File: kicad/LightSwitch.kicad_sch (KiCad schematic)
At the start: 33 parts, among them J1 Screw_Terminal_01x02, J2 Conn_01x06_Female, J3 Conn_ARM_JTAG_SWD_10, J4 Conn_ARM_JTAG_SWD_10, Q1 MMBT2222A, Q2 MMBT2222A, SW1 SW_Push_LED, SW2 SW_Push_LED, SW3 SW_Push_LED, SW4 SW_Push_LED, SW5 SW_Push_LED, U1 LM2936-3.0, U2 SHT35-DIS, U3 E73-2G4M08S1C, U4 MX25R3235FM2xx0, Y1 32.768kHz

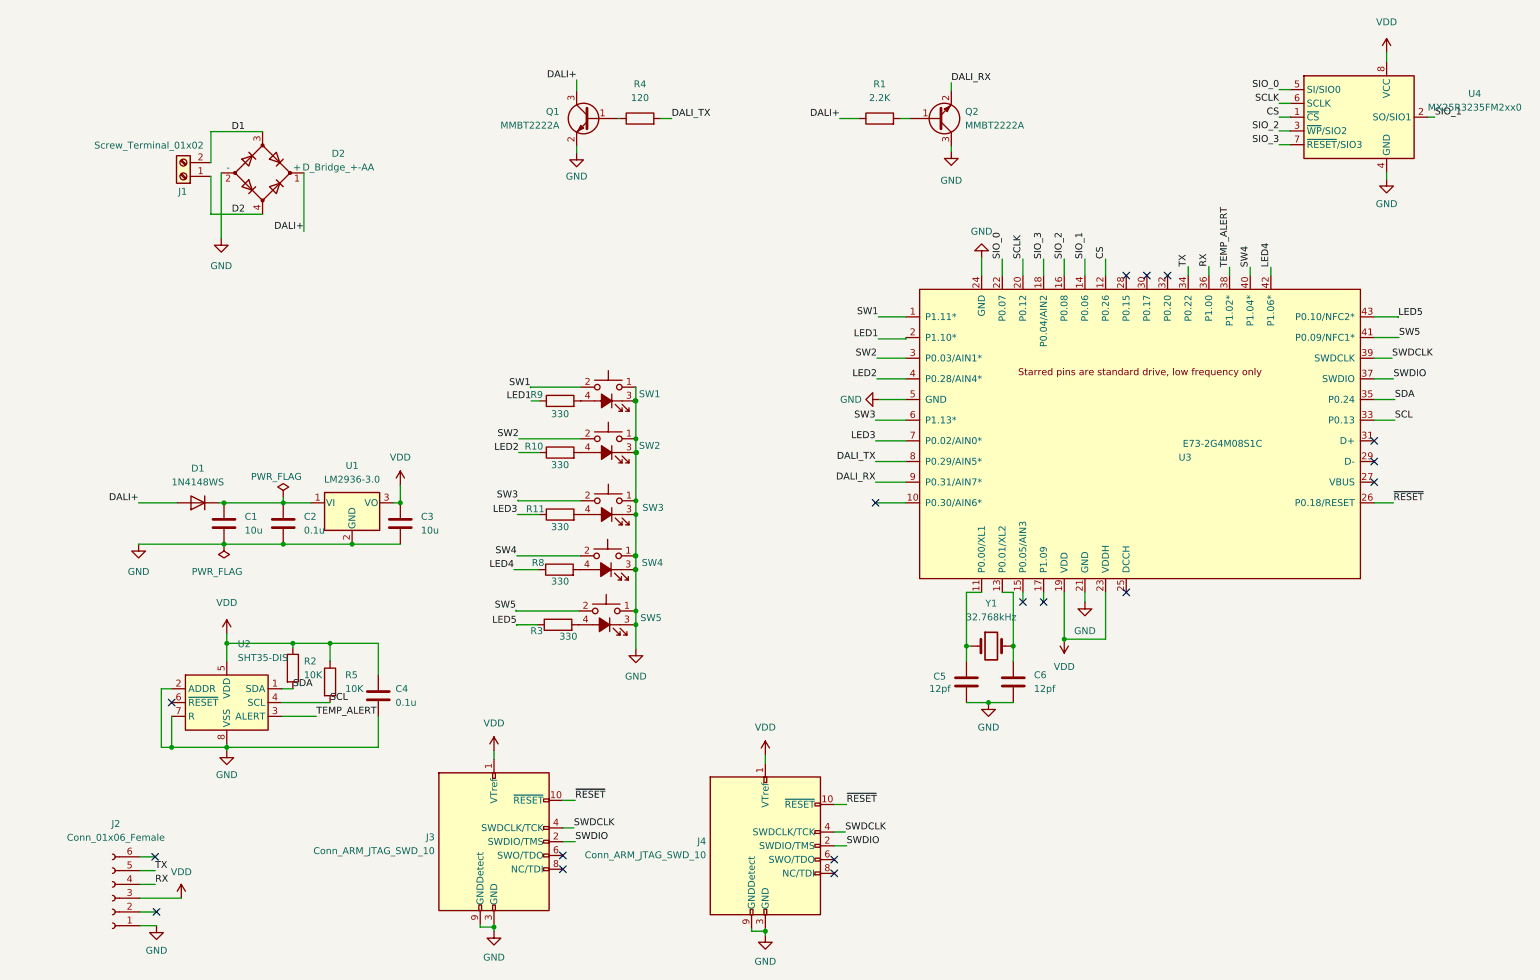
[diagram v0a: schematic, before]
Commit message: latect schematic
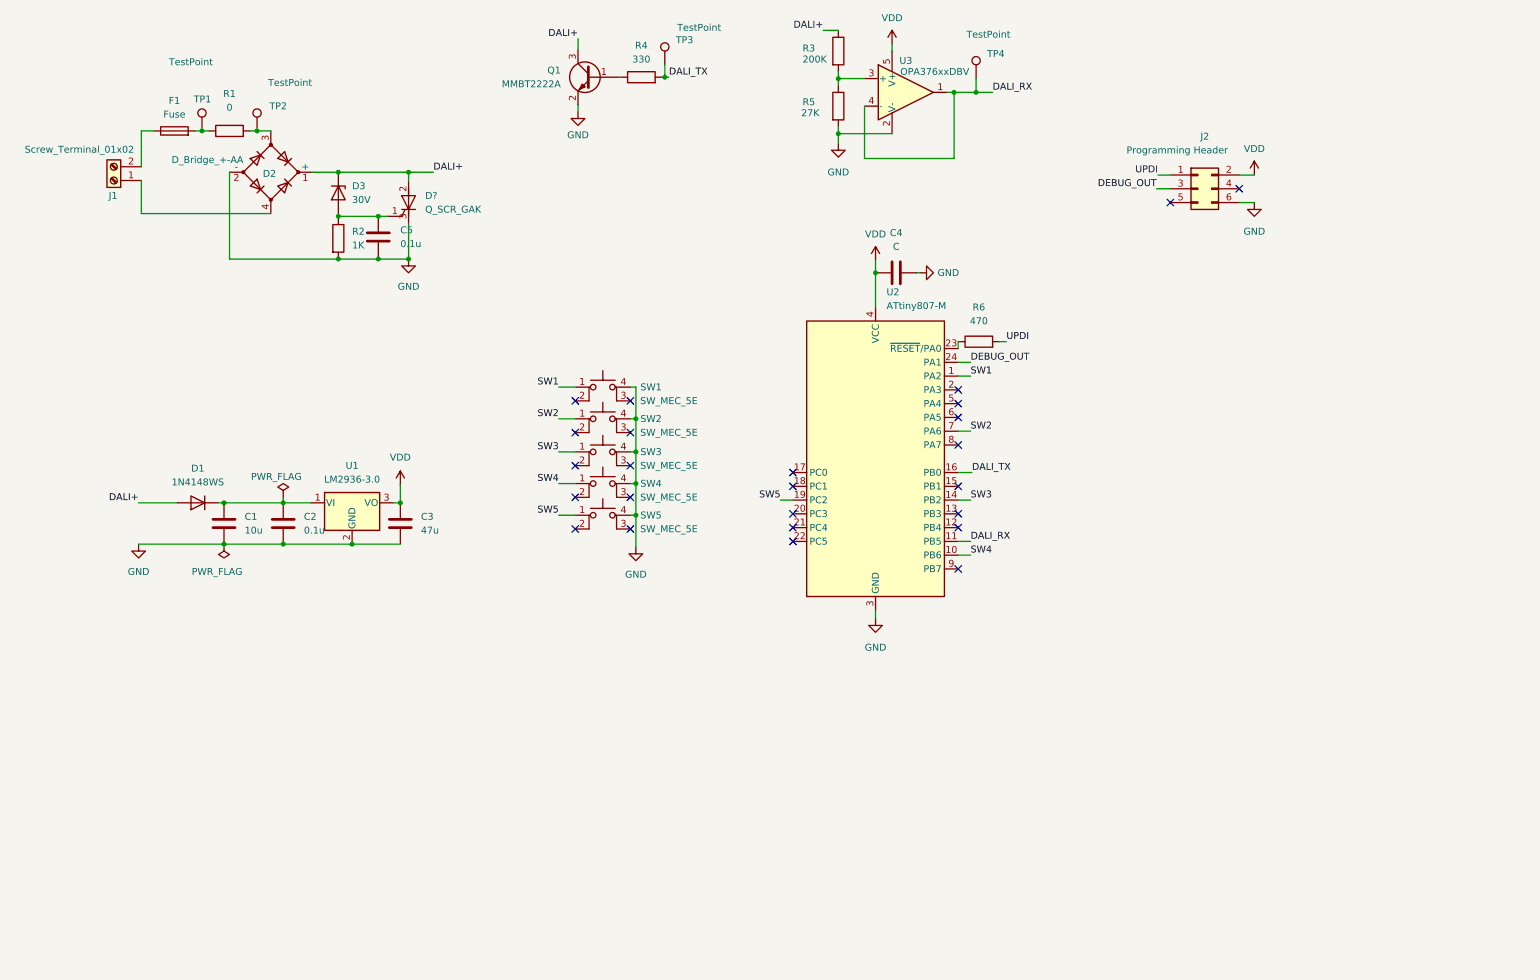
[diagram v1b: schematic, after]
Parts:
- removed C6: 12pf, Capacitor_SMD:C_0805_2012Metric, symbol Device:C
- removed J2: Conn_01x06_Female, Connector_PinSocket_2.54mm:PinSocket_1x06_P2.54mm_Vertical, symbol Connector:Conn_01x06_Female
- removed J3: Conn_ARM_JTAG_SWD_10, Connector_PinHeader_1.27mm:PinHeader_2x05_P1.27mm_Vertical_SMD, symbol Connector:Conn_ARM_JTAG_SWD_10
- removed J4: Conn_ARM_JTAG_SWD_10, Connector:Tag-Connect_TC2050-IDC-NL_2x05_P1.27mm_Vertical, symbol Connector:Conn_ARM_JTAG_SWD_10
- removed Q2: MMBT2222A, Package_TO_SOT_SMD:SOT-23, symbol Device:Q_NPN_BEC
- removed R10, R11, R8, R9: 330, Resistor_SMD:R_0805_2012Metric, symbol Device:R
- removed SW1, SW2, SW3, SW4, SW5: SW_Push_LED, LocalProject:LED Pushbutton, symbol Switch:SW_Push_LED
- removed U2: SHT35-DIS, Sensor_Humidity:Sensirion_DFN-8-1EP_2.5x2.5mm_P0.5mm_EP1.1x1.7mm, symbol Sensor_Humidity:SHT35-DIS
- removed U3: E73-2G4M08S1C, E73-2G4M08S1C:E73-2G4M08S1C, symbol CDEbyte E73-2G4M08S1C:E73-2G4M08S1C
- removed U4: MX25R3235FM2xx0, Package_SO:SOP-8_5.28x5.23mm_P1.27mm, symbol Memory_Flash:MX25R3235FM2xx0
- removed Y1: 32.768kHz, Crystal:Crystal_SMD_3215-2Pin_3.2x1.5mm, symbol Device:Crystal
- added D3: 30V, symbol Device:D_Zener
- added D?: Q_SCR_GAK, symbol Device:Q_SCR_GAK
- added F1: Fuse, symbol Device:Fuse
- added J2: Programming Header, symbol Connector_Generic:Conn_02x03_Odd_Even
- added R6: 470, Connector:Tag-Connect_TC2030-IDC-NL_2x03_P1.27mm_Vertical, symbol Device:R
- added SW1, SW2, SW3, SW4, SW5: SW_MEC_5E, symbol Switch:SW_MEC_5E
- added TP1, TP2, TP3, TP4: TestPoint, symbol Connector:TestPoint
- added U2: ATtiny807-M, Package_DFN_QFN:QFN-24-1EP_4x4mm_P0.5mm_EP2.6x2.6mm, symbol MCU_Microchip_ATtiny:ATtiny807-M
- added U3: OPA376xxDBV, Package_TO_SOT_SMD:SOT-23-5, symbol Amplifier_Operational:OPA376xxDBV
- C3: value 10u -> 47u
- C4: value 0.1u -> C
- C5: value 12pf -> 0.1u; footprint Capacitor_SMD:C_0805_2012Metric -> (none)
- R1: value 2.2K -> 0; footprint Resistor_SMD:R_0805_2012Metric -> (none)
- R2: value 10K -> 1K; footprint Resistor_SMD:R_0805_2012Metric -> (none)
- R3: value 330 -> 200K; footprint Resistor_SMD:R_0805_2012Metric -> (none)
- R4: value 120 -> 330
- R5: value 10K -> 27K; footprint Resistor_SMD:R_0805_2012Metric -> (none)
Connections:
- net LED5 is gone; now on net DALI+: R3.1
- net SCL is gone; now on net GND: R5.2
- net SDA is gone; now on net GND: R2.2
- net DALI+: now also D3.1 (K), D?.2 (A); no longer R1.1
- net DALI_RX: now also TP4.1, U2.11 (PB5), U3.1, U3.4 (-)
- net DALI_TX: now also TP3.1, U2.16 (PB0)
- net GND: now also C4.2, D?.3 (K), J2.6 (Pin_6), SW1.4 (A), SW2.4 (A), SW3.4 (A), SW4.4 (A), SW5.4 (A), U2.25 (GND), U2.3 (GND), U3.2 (V-); no longer C4.1
- net SW1: now also SW1.1, U2.1 (PA2)
- net SW2: now also SW2.1, U2.7 (PA6)
- net SW3: now also SW3.1, U2.14 (PB2)
- net SW4: now also SW4.1, U2.10 (PB6)
- net SW5: now also SW5.1, U2.19 (PC2)
- net VDD: now also C4.1, J2.2 (Pin_2), U2.4 (VCC), U3.5 (V+); no longer C4.2, R2.1, R5.1
- net at R3.2: now also R5.1, U3.3 (+)
- net at C5.1: now also R2.1, D3.2 (A), D?.1 (G)
- net at R1.2: now also D2.3, TP2.1
- net D1: no longer names the net of J1.2 (Pin_2)
- net D1: now also F1.1; no longer D2.3
- net D2: no longer names the net of D2.4, J1.1 (Pin_1)
- new net: F1.2, R1.1, TP1.1
- new net: R6.1, U2.23 (~{RESET}/PA0)
- new net DEBUG_OUT: J2.3 (Pin_3), U2.24 (PA1)
- new net UPDI: J2.1 (Pin_1), R6.2
- no-connect marks 17 -> 25
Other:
- moved on the sheet: D2, J1, Q1, R4
